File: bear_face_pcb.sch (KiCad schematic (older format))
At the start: 201 parts, among them J1 GT-USB-7010EN, J2 Conn_02x03_Odd_Even, SW1 RESET, U1 ATmega32U4-AU, U2 SRV05-4, Y1 16MHz

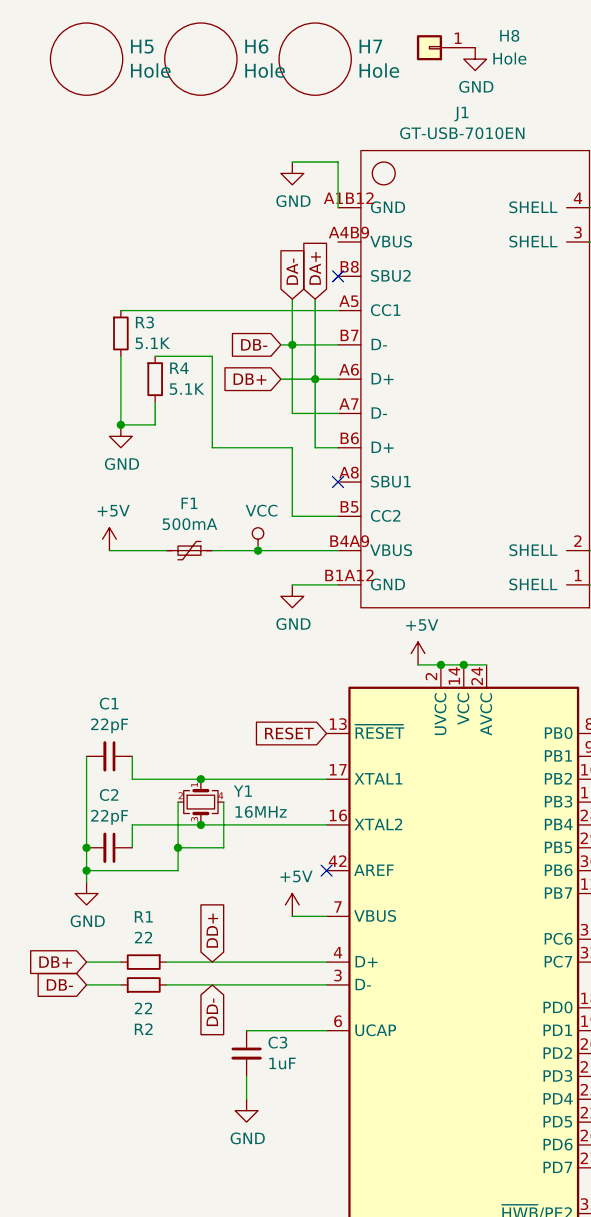
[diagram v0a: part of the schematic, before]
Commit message: ready for JLC, routing/place tweaks
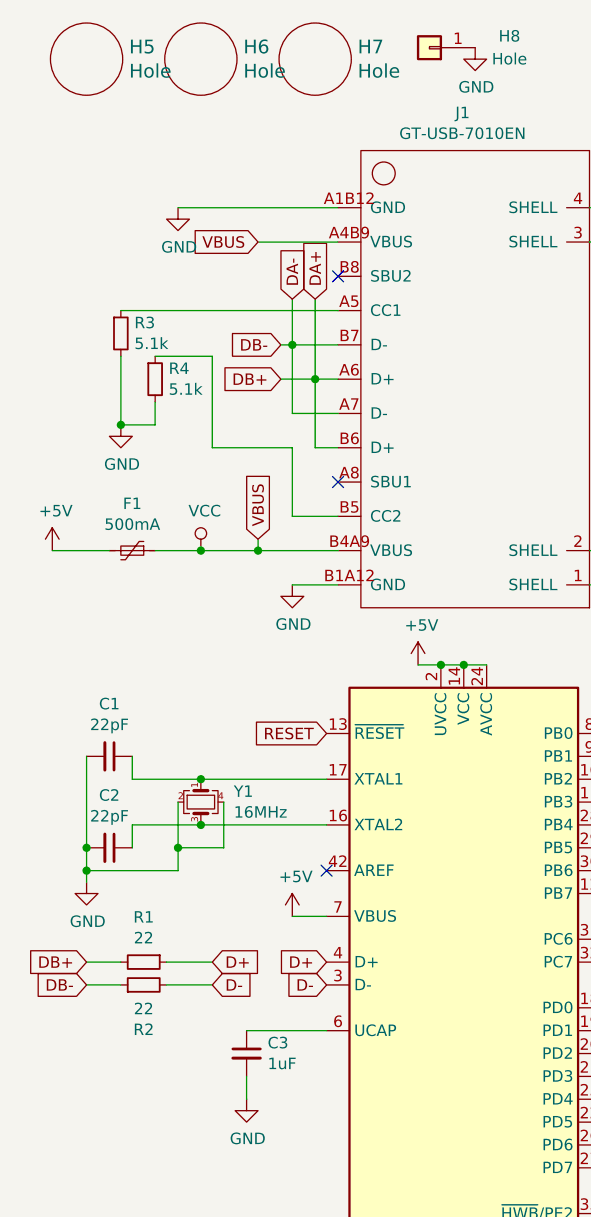
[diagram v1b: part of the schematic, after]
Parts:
- C1, C2: LCSC (none) -> C1804; LCSC# C1804 -> (none)
- C3: LCSC (none) -> C28323; LCSC# C28323 -> (none)
- C4, C5, C6: LCSC (none) -> C49678; LCSC# C49678 -> (none)
- C7: LCSC (none) -> C15850; LCSC# C15850 -> (none)
- D1, D10, D11, D12, D13, D14, D15, D16, D17, D18, D19, D2, D20, D21, D22, D23, D24, D25, D26, D27, D28, D29, D3, D30, D31, D32, D33, D34, D35, D36, D37, D38, D39, D4, D40, D41, D42, D43, D44, D45, D46, D47, D48, D49, D5, D50, D51, D52, D53, D54, D55, D56, D57, D58, D59, D6, D60, D61, D62, D63, D64, D65, D66, D67, D68, D69, D7, D70, D71, D72, D73, D74, D75, D76, D77, D78, D79, D8, D80, D81, D82, D83, D84, D85, D9: LCSC (none) -> C81598; LCSC# C81598 -> (none)
- F1: LCSC (none) -> C70076; LCSC# C70076 -> (none)
- J1: LCSC (none) -> C3001297; LCSC# C3001297 -> (none)
- R1, R2: LCSC (none) -> C17561
- R3, R4: value 5.1K -> 5.1k; LCSC (none) -> C2907269
- R5: LCSC (none) -> C17710; LCSC# C17710 -> (none)
- R6, R7: LCSC (none) -> C17414; LCSC# C17414 -> (none)
- U1: LCSC (none) -> C44854; LCSC# C44854 -> (none)
- U2: LCSC (none) -> C85364; LCSC# C85364 -> (none)
- Y1: LCSC (none) -> C13738; LCSC# C13738 -> (none)
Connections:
- net VCC: now also J1.A4B9 (VBUS)
- net DD+ renamed D+
- net DD- renamed D-
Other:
- moved on the sheet: F1
